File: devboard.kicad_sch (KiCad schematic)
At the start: 0 parts

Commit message: devlog 03
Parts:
- added C1: 18p, Capacitor_SMD:C_0402_1005Metric, symbol Device:C
- added C10: 4u7, Capacitor_SMD:C_0402_1005Metric, symbol Device:C
- added C11, C15, C3, C6, C7, C8, C9: 100n, Capacitor_SMD:C_0402_1005Metric, symbol Device:C
- added C12: 2u2, Capacitor_SMD:C_0402_1005Metric, symbol Device:C
- added C13, C5: 1u, Capacitor_SMD:C_0402_1005Metric, symbol Device:C
- added C14, C4: 10u, Capacitor_SMD:C_0402_1005Metric, symbol Device:C
- added C2: GND, Capacitor_SMD:C_0402_1005Metric, symbol Device:C
- added D1: USBLC6-2SC6, Package_TO_SOT_SMD:SOT-23-6, symbol Power_Protection:USBLC6-2SC6
- added J1: USB-C, Connector_USB:USB_C_Receptacle_GCT_USB4105-xx-A_16P_TopMnt_Horizontal, symbol Connector:USB_C_Receptacle_USB2.0_16P
- added J2: microSD, symbol Connector:Micro_SD_Card_Det1
- added J3: SWD, symbol Connector_Generic:Conn_01x04
- added J4: GPIO-A, symbol Connector_Generic:Conn_01x08
- added J5: GPIO-B, symbol Connector_Generic:Conn_01x08
- added J6: GPIO-C, symbol Connector_Generic:Conn_01x08
- added J7: DBG-PWR, symbol Connector_Generic:Conn_01x08
- added LED1: GREEN, LED_SMD:LED_0603_1608Metric, symbol Device:LED
- added R1, R2, R6: 10k, Resistor_SMD:R_0402_1005Metric, symbol Device:R
- added R10, R11, R12, R13, R9: 47k, Resistor_SMD:R_0402_1005Metric, symbol Device:R
- added R3, R4: 5k1, Resistor_SMD:R_0402_1005Metric, symbol Device:R
- added R5: 1k, Resistor_SMD:R_0402_1005Metric, symbol Device:R
- added R8: 10R, Resistor_SMD:R_0402_1005Metric, symbol Device:R
- added SW1: RESET, symbol Switch:SW_Push
- added SW2: BOOT0, symbol Switch:SW_Push
- added SW3: USER, symbol Switch:SW_Push
- added U1: STM32F411CEU6, Package_DFN_QFN:QFN-48-1EP_7x7mm_P0.5mm_EP5.15x5.15mm, symbol MCU_ST_STM32F4:STM32F411CEUx
- added U2: AP2112K-3.3, Package_TO_SOT_SMD:SOT-23-5, symbol Regulator_Linear:AP2112K-3.3
- added Y1: 25MHz, symbol Device:Crystal
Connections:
- new net 3v3: C10.1, C13.1, C14.1, C15.1, C6.1, C7.1, C8.1, C9.1, J2.4 (VDD), J3.1 (Pin_1), J6.7 (Pin_7), J7.1 (Pin_1), R1.1, R10.2, R11.2, R12.2, R13.2, R8.1, R9.2, SW2.1, SW3.1, U1.1 (VBAT), U1.24 (VDD), U1.36 (VDD), U1.48 (VDD), U2.5 (VOUT)
- new net BOOT0_NET: J7.7 (Pin_7), R2.1, SW2.2, U1.44 (BOOT0)
- new net CC1_NET: J1.A5 (CC1), R3.1
- new net CC2_NET: J1.B5 (CC2), R4.1
- new net GND: C1.2, C10.2, C11.2, C12.2, C13.2, C14.2, C15.2, C2.2, C3.2, C4.2, C5.2, C6.2, C7.2, C8.2, C9.2, D1.2 (GND), J1.A1 (GND), J1.A12 (GND), J1.B1 (GND), J1.B12 (GND), J1.SH (SHIELD), J2.6 (VSS), J2.SH (SHIELD), J3.4 (Pin_4), J6.8 (Pin_8), J7.4 (Pin_4), LED1.1 (K), R2.2, R3.2, R4.2, R6.2, SW1.1, U1.23 (VSS), U1.35 (VSS), U1.47 (VSS), U1.49 (VSS), U1.8 (VSSA), U2.2 (GND)
- new net LED_A: LED1.2 (A), R5.2
- new net LED_NET: R5.1, U1.2 (PC13)
- new net NRST: C3.1, J7.5 (Pin_5), R1.2, SW1.2, U1.7 (NRST)
- new net OSC_IN: C1.1, U1.5 (PH0), Y1.1
- new net OSC_OUT: C2.1, U1.6 (PH1), Y1.2
- new net PA1: J4.1 (Pin_1), U1.11 (PA1)
- new net PA10: J5.1 (Pin_1), U1.31 (PA10)
- new net PA15: J5.2 (Pin_2), U1.38 (PA15)
- new net PA2: J4.2 (Pin_2), U1.12 (PA2)
- new net PA3: J4.3 (Pin_3), U1.13 (PA3)
- new net PA4: J4.4 (Pin_4), U1.14 (PA4)
- new net PA5: J4.5 (Pin_5), U1.15 (PA5)
- new net PA6: J4.6 (Pin_6), U1.16 (PA6)
- new net PA7: J4.7 (Pin_7), U1.17 (PA7)
- new net PA8: J4.8 (Pin_8), U1.29 (PA8)
- new net PB0: J5.3 (Pin_3), U1.18 (PB0)
- new net PB1: J5.4 (Pin_4), U1.19 (PB1)
- new net PB10: J6.4 (Pin_4), U1.21 (PB10)
- new net PB2: J5.5 (Pin_5), U1.20 (PB2)
- new net PB3: J5.6 (Pin_6), U1.39 (PB3)
- new net PB4: J5.7 (Pin_7), U1.40 (PB4)
- new net PB5: J5.8 (Pin_8), U1.41 (PB5)
- new net PB6: J6.1 (Pin_1), U1.42 (PB6)
- new net PB7: J6.2 (Pin_2), U1.43 (PB7)
- new net PB9: J6.3 (Pin_3), U1.46 (PB9)
- new net PC14: J6.5 (Pin_5), U1.3 (PC14)
- new net PC15: J6.6 (Pin_6), U1.4 (PC15)
- new net SD_CD: J2.9 (DET), R11.1, U1.45 (PB8)
- new net SD_CS: J2.2 (DAT3/CD), R9.1, U1.25 (PB12)
- new net SD_DAT1: J2.8 (DAT1), R12.1
- new net SD_DAT2: J2.1 (DAT2), R13.1
- new net SD_MISO: J2.7 (DAT0), R10.1, U1.27 (PB14)
- new net SD_MOSI: J2.3 (CMD), U1.28 (PB15)
- new net SD_SCK: J2.5 (CLK), U1.26 (PB13)
- new net SWCLK: J3.3 (Pin_3), J7.3 (Pin_3), U1.37 (PA14)
- new net SWDIO: J3.2 (Pin_2), J7.2 (Pin_2), U1.34 (PA13)
- new net USB_DM: D1.3 (I/O2), D1.4 (I/O2), J1.A7 (D-), J1.B7 (D-), U1.32 (PA11)
- new net USB_DP: D1.1 (I/O1), D1.6 (I/O1), J1.A6 (D+), J1.B6 (D+), U1.33 (PA12)
- new net USER_BTN: J7.8 (Pin_8), R6.1, SW3.2, U1.10 (PA0)
- new net VBUS: C4.1, C5.1, D1.5 (VBUS), J1.A4 (VBUS), J1.A9 (VBUS), J1.B4 (VBUS), J1.B9 (VBUS), J7.6 (Pin_6), U1.30 (PA9), U2.1 (VIN), U2.3 (EN)
- new net VCAP: C12.1, U1.22 (VCAP1)
- new net VDDA: C11.1, R8.2, U1.9 (VDDA)
- no-connect marks 0 -> 2

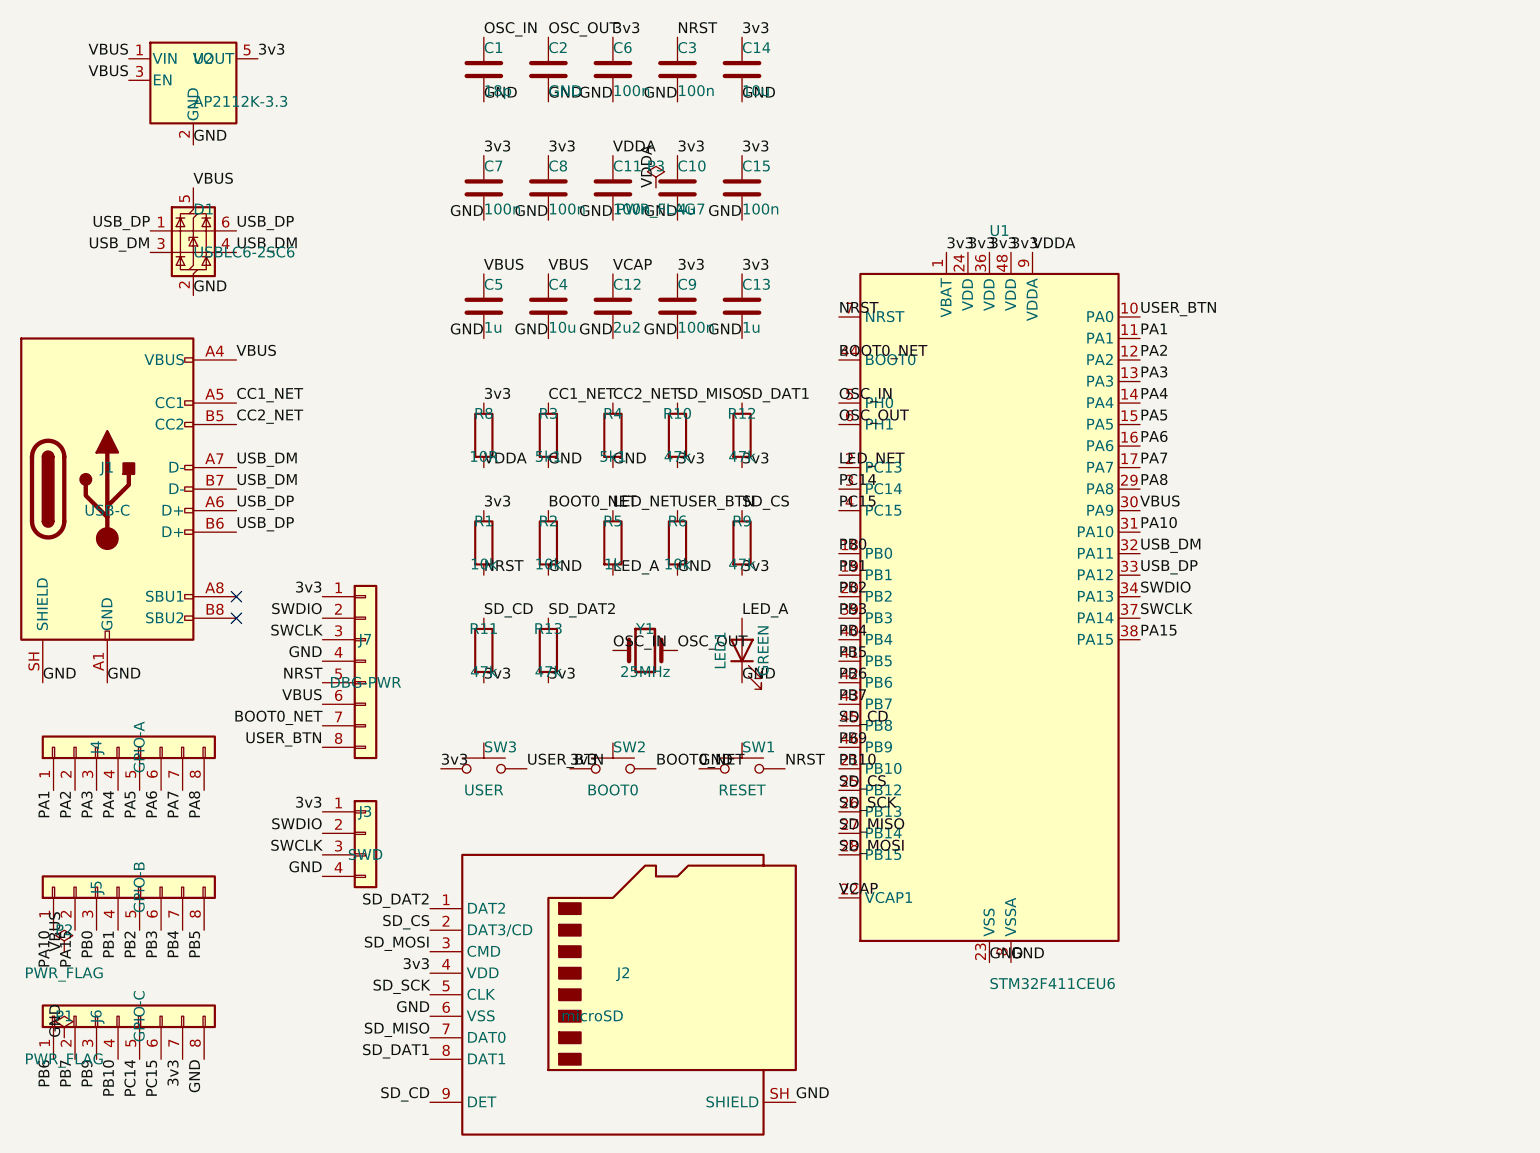
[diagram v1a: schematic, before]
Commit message: pcb routing
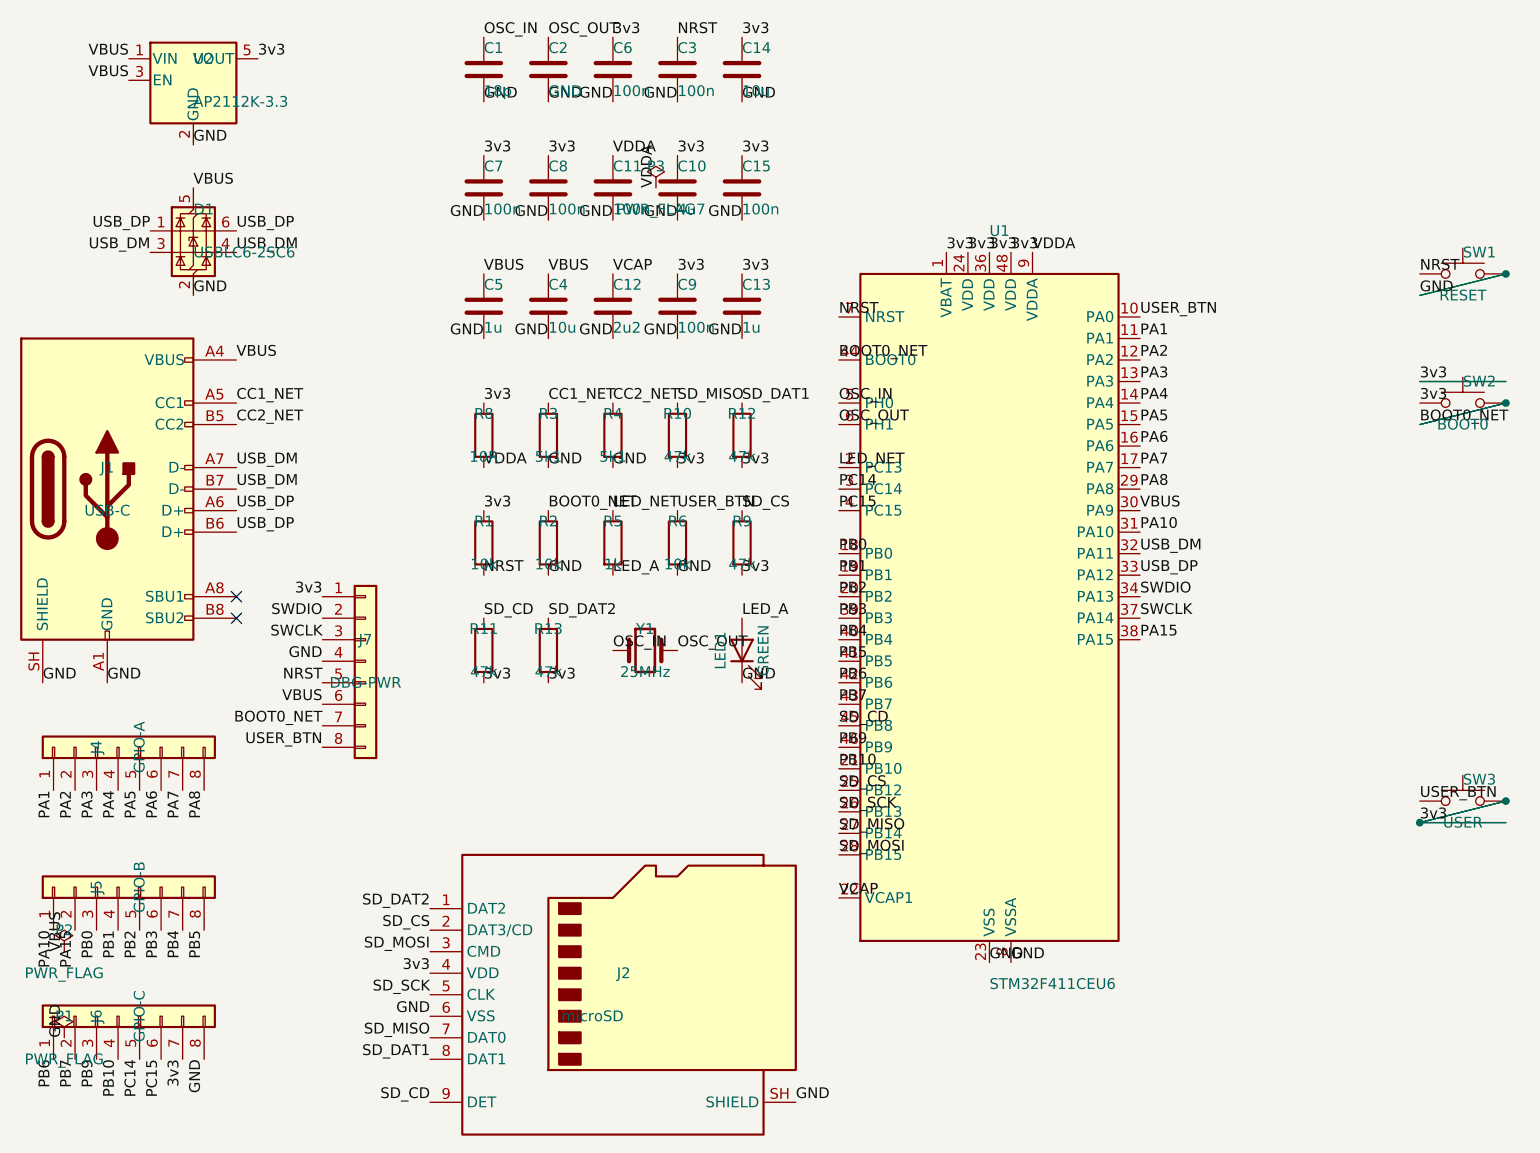
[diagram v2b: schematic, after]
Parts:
- removed J3: SWD, symbol Connector_Generic:Conn_01x04
- J2: footprint (none) -> Connector_Card:microSD_HC_Hirose_DM3AT-SF-PEJM5
- J4, J5, J6, J7: footprint (none) -> Connector_PinHeader_2.54mm:PinHeader_1x08_P2.54mm_Vertical
- SW1, SW2, SW3: footprint (none) -> Button_Switch_SMD:SW_SPST_PTS645Sx43SMTR92
- Y1: footprint (none) -> Crystal:Crystal_SMD_Abracon_ABM3-2Pin_5.0x3.2mm
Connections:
- net 3v3: now also SW3.2; no longer SW3.1
- net GND: now also SW1.2; no longer SW1.1
- net NRST: now also SW1.1; no longer SW1.2
- net USER_BTN: now also SW3.1; no longer SW3.2

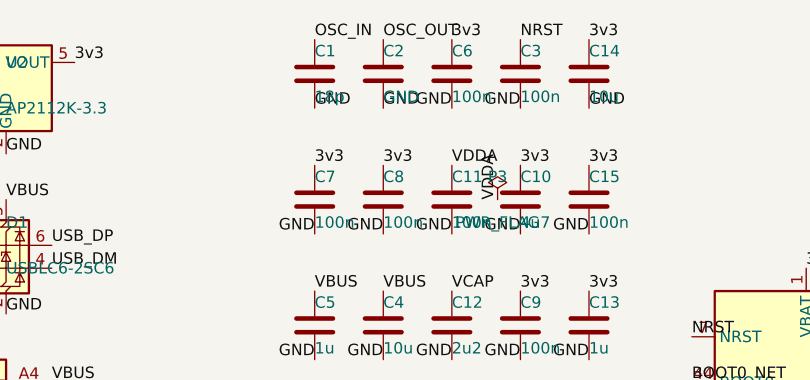
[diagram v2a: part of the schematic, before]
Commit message: devlog 05
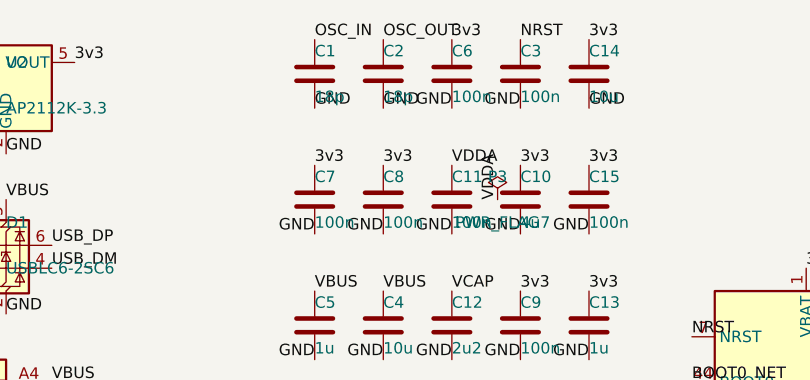
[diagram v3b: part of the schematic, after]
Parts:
- C2: value GND -> 18p
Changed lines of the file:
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@@
 			)
 		)
-		(property "Value" "GND"
+		(property "Value" "18p"
 			(at 87.63 38.1 0)
 			(show_name no)

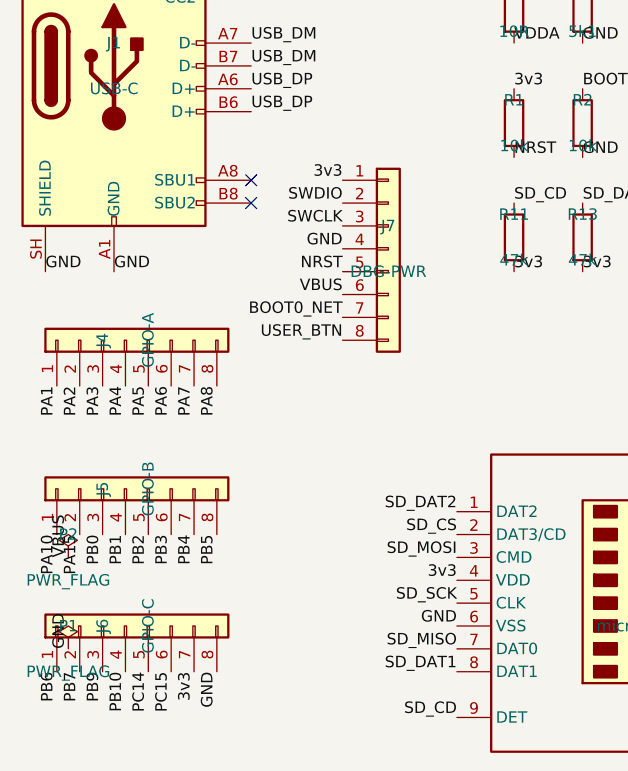
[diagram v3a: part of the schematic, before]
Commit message: devlog 07
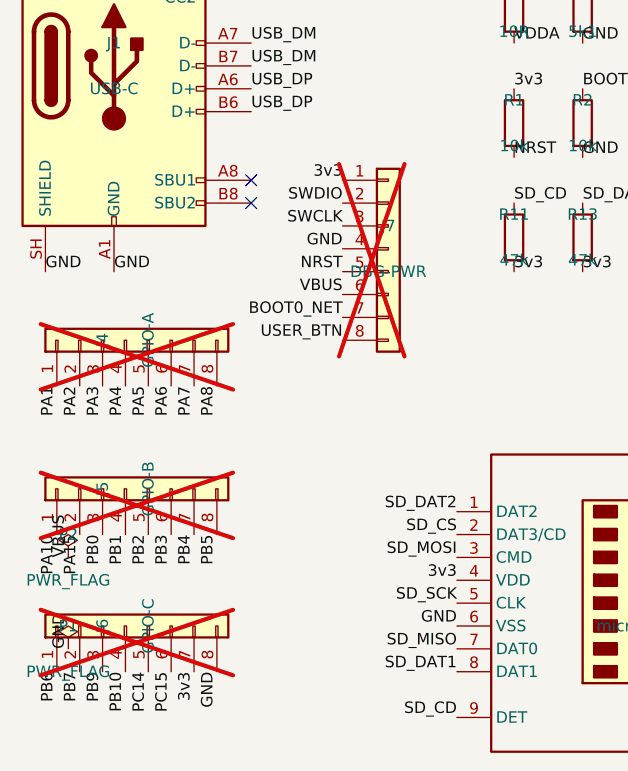
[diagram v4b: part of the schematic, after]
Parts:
- J4, J5, J6, J7: now not fitted
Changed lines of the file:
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@@
 		(on_board yes)
 		(in_pos_files yes)
-		(dnp no)
+		(dnp yes)
 		(property "Reference" "J5"
 			(at 34.29 132.08 0)
@@
 		(on_board yes)
 		(in_pos_files yes)
-		(dnp no)
+		(dnp yes)
 		(property "Reference" "J6"
 			(at 34.29 147.32 0)
@@
 		(on_board yes)
 		(in_pos_files yes)
-		(dnp no)
+		(dnp yes)
 		(property "Reference" "J4"
 			(at 34.29 115.57 0)
@@
 		(on_board yes)
 		(in_pos_files yes)
-		(dnp no)
+		(dnp yes)
 		(property "Reference" "J7"
 			(at 66.04 102.87 0)
